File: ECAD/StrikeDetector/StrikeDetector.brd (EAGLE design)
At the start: 30 x 55 mm, 32 parts, among them J1 10118193-0001LF, U1 MMBT2222A-7-F, U2 MMBT2222A-7-F, U3 LSM9DS1TR, U4 ESP32-WROOM-32, U6 AP2112K-3.3TRG1

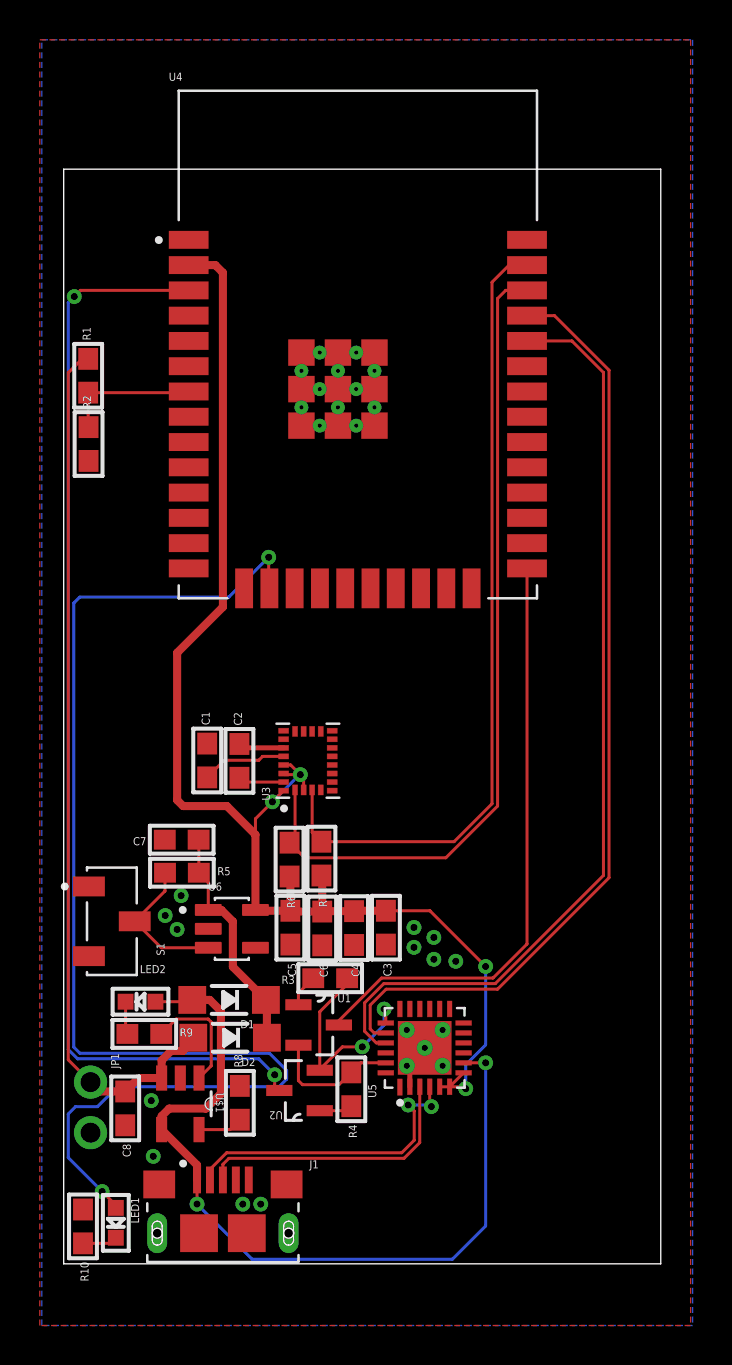
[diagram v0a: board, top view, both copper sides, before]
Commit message: Updated PCB Design
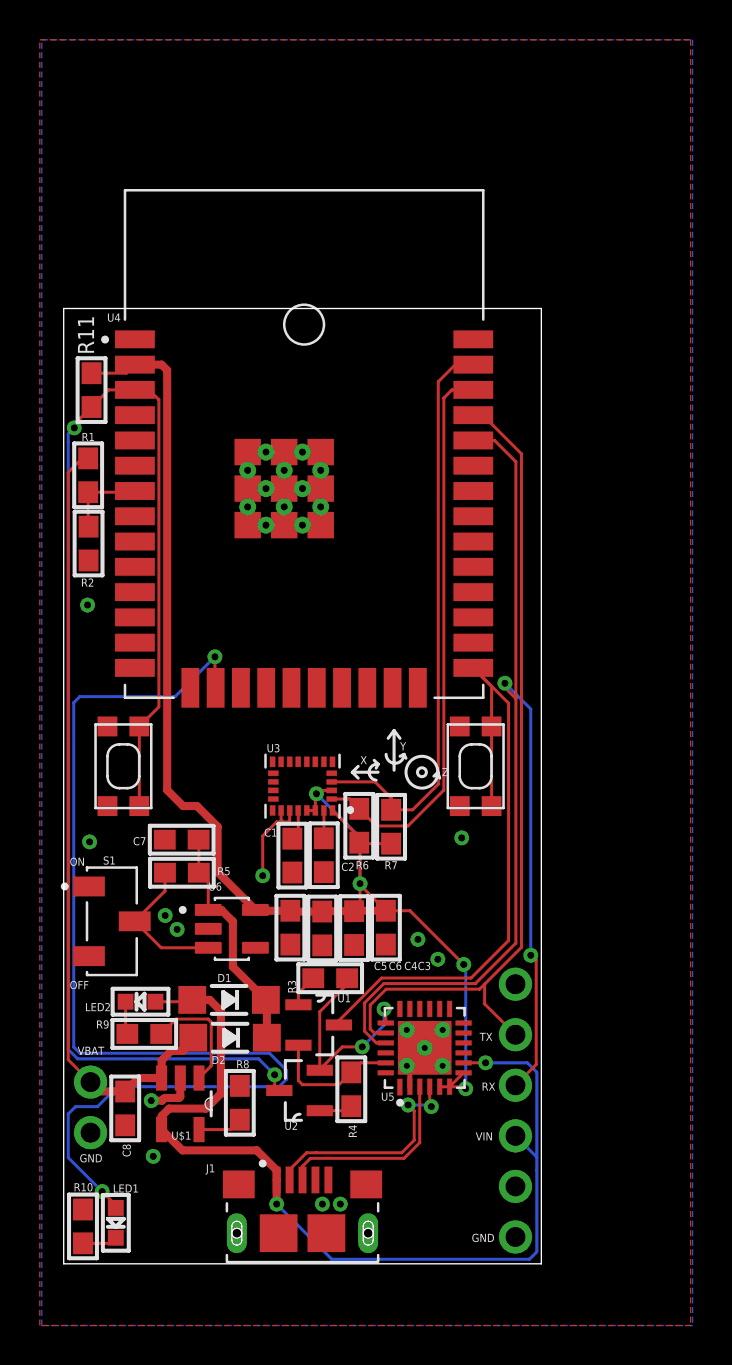
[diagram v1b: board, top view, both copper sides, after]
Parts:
- added JP3: (no value), microbuilder:1X06_ROUND
- added R11: 100kΩ, microbuilder:0603
- added SW1, SW2: KMR211GLFS, adafruit:KMR2
- moved C1 6.42 mm to (11.5, 20.5), turned to 270 degrees
- moved C2 6.36 mm to (13.1, 20.5), turned to 270 degrees
- moved U4 5.68 mm to (12.1, 41.2)
- moved R1 5.00 mm to (1.23, 39.6)
- moved R2 5.00 mm to (1.25, 36.2)
- moved J1 4.00 mm to (12.0, 1.54)
- moved R6 3.89 mm to (14.8, 22.0)
- moved R7 3.85 mm to (16.4, 22.0)
- moved U3 1.31 mm to (12.0, 24.0), turned to 180 degrees
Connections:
- new net N$13: JP3.2
- new net N$17: JP3.6
- net 3.3V: now also R11.2
- net GND: now also JP3.1, SW1.1, SW1.3, SW2.1, SW2.3
- net GPIO0: now also SW2.2, SW2.4
- net RESET: now also R11.1, SW1.2, SW1.4
- net RXD0: now also JP3.4
- net TXD0: now also JP3.5
- net VIN: now also JP3.3
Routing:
- net RESET: track 55.6 -> 69.3 mm
- net RXD0: track 47.2 -> 60.7 mm, vias 0 -> 2
- net SCL: track 41.8 -> 28.3 mm
- net SDA: track 40.5 -> 29.2 mm
- net GPIO13: track 63.7 -> 56.0 mm
- net VIN: track 42.0 -> 48.9 mm
- net TXD0: track 47.5 -> 42.1 mm
- net VBAT: track 44.5 -> 39.5 mm
- net GND: track 3.62 -> 8.49 mm
- net N$2: track 13.9 -> 9.87 mm
- net N$3: track 15.5 -> 11.5 mm
- net 3.3V: track 74.3 -> 70.6 mm
- net N$1: track 4.28 -> 1.54 mm
- net BAT_VAL: track 6.86 -> 4.16 mm
- net GPIO0: track 30.1 -> 32.2 mm
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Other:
- board size 30 x 55 mm -> 24 x 48 mm
- board text added: "GND"
- board text added: "OFF"
- board text added: "ON"
- board text added: "RX"
- board text added: "TX"
- board text added: "VBAT"
- board text added: "VIN"
- board text added: "X"
- board text added: "Y"
- board text added: "Z"
